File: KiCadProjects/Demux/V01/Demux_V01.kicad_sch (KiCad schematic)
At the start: 34 parts, among them J1 alimentacao analogica, J10 +3.3Vmux, J11 -9Vmux, J12 -5Vmux, J13 GNDmux, J14 conectorEletrodos, J15 conectorEletrodos, J2 sinais analogicos, J3 comunicacao / sinais digitais, J4 Conn_01x03, J5 Conn_01x02, J6 Conn_01x02, J7 Conn_01x02, J8 +9Vmux, J9 +5Vmux, U1A1 74HC4051, U1B1 74HC4051, U2 BluePill_STM32F103C, U2A2 74HC4051, U2B2 74HC4051, U3A3 74HC4051, U3B3 74HC4051, U4A4 74HC4051, U4B4 74HC4051, U5A1 74HC4051, U5B1 74HC4051

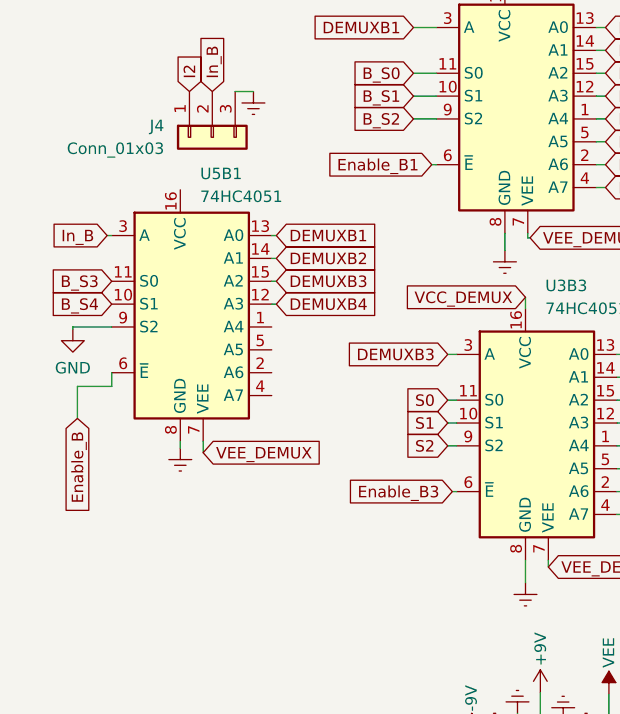
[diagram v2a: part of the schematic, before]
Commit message: correcao Vcc mux U5B1
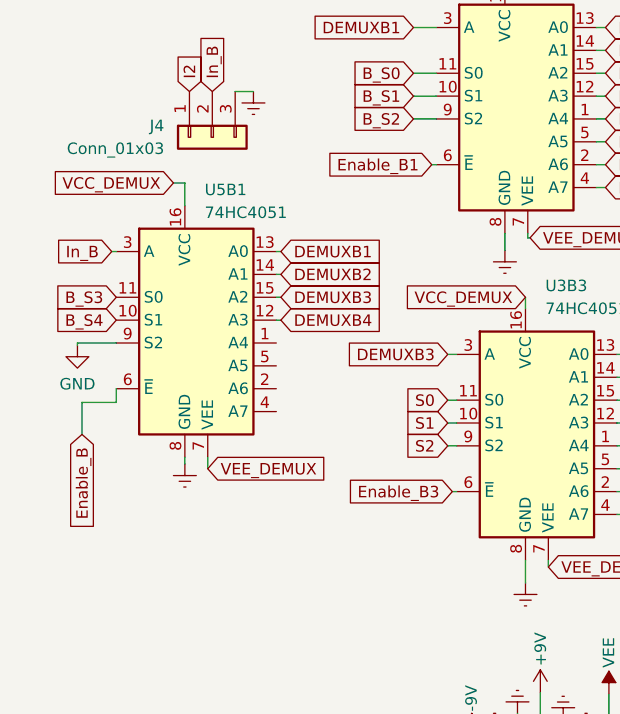
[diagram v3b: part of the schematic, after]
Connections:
- net VCC_DEMUX: now also U5B1.16 (VCC)
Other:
- moved on the sheet: U5B1
